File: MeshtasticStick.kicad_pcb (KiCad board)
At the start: 2 copper layers, 31 x 60 mm, 3 parts

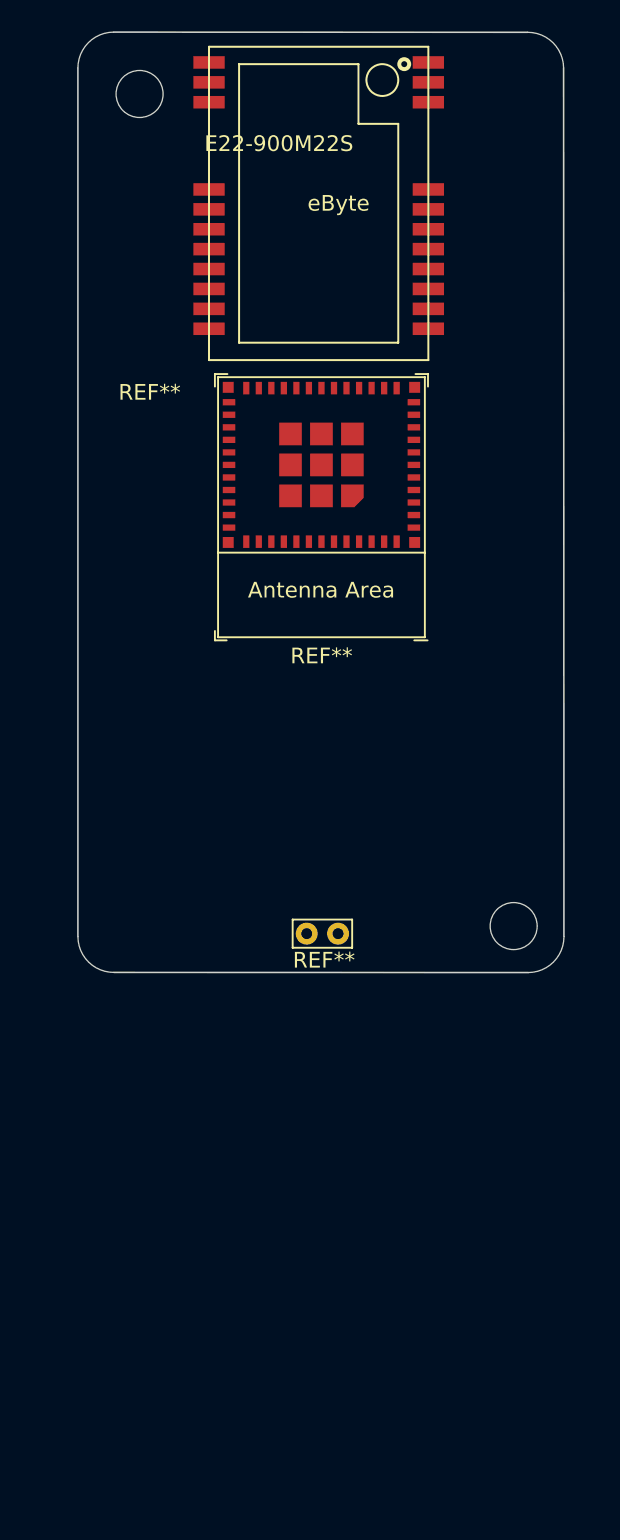
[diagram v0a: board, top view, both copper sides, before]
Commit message: ver1
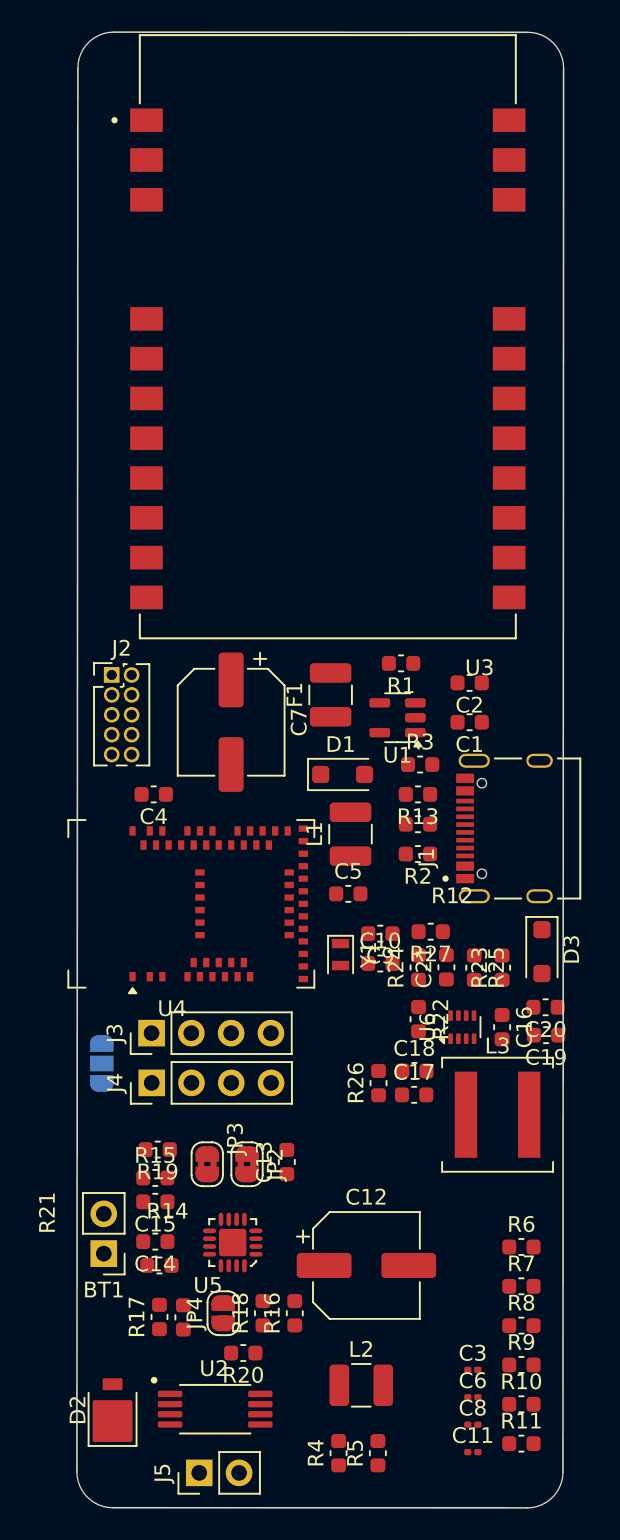
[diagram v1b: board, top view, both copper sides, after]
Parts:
- removed REF**: ESP32-PICO-MINI-02, PCM_Espressif:ESP32-PICO-MINI-02
- removed REF**: E22-900M22S, RF_Module:E22-900M22S
- removed REF**: TestPoint_Bridge_Pitch2.0mm_Drill0.7mm, TestPoint:TestPoint_Bridge_Pitch2.0mm_Drill0.7mm
- added BT1: Battery_Cell, Connector_PinHeader_2.54mm:PinHeader_1x02_P2.54mm_Vertical, F.Cu at (126.5, 146.8)
- added C1: 1uF, Capacitor_SMD:C_0603_1608Metric, F.Cu at (149.8, 112.9)
- added C10: 14p, Capacitor_SMD:C_0603_1608Metric, F.Cu at (144.1, 128.3)
- added C11: 1nF, Capacitor_SMD:C_0201_0603Metric, F.Cu at (150.0, 159.5)
- added C12: 47uF, Capacitor_SMD:CP_Elec_6.3x7.7, F.Cu at (143.3, 147.5)
- added C13: 10nF, Capacitor_SMD:C_0603_1608Metric, F.Cu at (138.2, 140.9)
- added C14: 4.7uF, Capacitor_SMD:C_0603_1608Metric, F.Cu at (129.8, 146.0)
- added C15: 1nF, Capacitor_SMD:C_0603_1608Metric, F.Cu at (129.8, 143.5)
- added C16: 0.1uF, Capacitor_SMD:C_0603_1608Metric, F.Cu at (151.9, 132.3)
- added C17: 10uF, Capacitor_SMD:C_0603_1608Metric, F.Cu at (146.3, 136.7)
- added C18: 0.1uF, Capacitor_SMD:C_0603_1608Metric, F.Cu at (146.3, 135.1)
- added C19: 22uF, Capacitor_SMD:C_0603_1608Metric, F.Cu at (154.7, 132.8)
- added C2: 1uF, Capacitor_SMD:C_0603_1608Metric, F.Cu at (149.8, 110.4)
- added C20: 22uF, Capacitor_SMD:C_0603_1608Metric, F.Cu at (154.7, 131.1)
- added C21: 22nF, Capacitor_SMD:C_0603_1608Metric, F.Cu at (148.4, 128.5)
- added C3: 1uF, Capacitor_SMD:C_0201_0603Metric, F.Cu at (150.0, 154.2)
- added C4: 4.7uF, Capacitor_SMD:C_0603_1608Metric, F.Cu at (129.7, 117.5)
- added C5: 4.7uF, Capacitor_SMD:C_0603_1608Metric, F.Cu at (142.1, 123.8)
- added C6: 1nF, Capacitor_SMD:C_0201_0603Metric, F.Cu at (150.0, 156.0)
- added C7: 100uF, Capacitor_SMD:CP_Elec_6.3x7.7, F.Cu at (134.6, 112.9)
- added C8: 10uF, Capacitor_SMD:C_0201_0603Metric, F.Cu at (150.0, 157.7)
- added C9: 14p, Capacitor_SMD:C_0603_1608Metric, F.Cu at (144.1, 126.4)
- added D1: MBR120VLSFT1G, Diode_SMD:D_SOD-123F, F.Cu at (141.7, 116.2)
- added D2: SMM4F5.0A, Diode_SMD:D_SMP_DO-220AA, F.Cu at (127.1, 156.8)
- added D3: MBR120VLSFT1G, Diode_SMD:D_SOD-123F, F.Cu at (154.5, 127.5)
- added F1: Fuse, Fuse:Fuse_1210_3225Metric, F.Cu at (141.0, 111.1)
- added J1: TYPE-C-31-M-12, TYPE-C-31-M-12 footprint:HRO_TYPE-C-31-M-12, F.Cu at (154.3, 119.7)
- added J2: Conn_02x05_Odd_Even, Connector_PinHeader_1.27mm:PinHeader_2x05_P1.27mm_Vertical, F.Cu at (127.0, 109.9)
- added J3: Conn_01x04, Connector_PinHeader_2.54mm:PinHeader_1x04_P2.54mm_Vertical, F.Cu at (129.5, 132.7)
- added J4: Conn_01x04, Connector_PinHeader_2.54mm:PinHeader_1x04_P2.54mm_Vertical, F.Cu at (129.6, 135.9)
- added J5: Conn_01x02, Connector_PinHeader_2.54mm:PinHeader_1x02_P2.54mm_Vertical, F.Cu at (132.6, 160.8)
- added JP1: SolderJumper_3_Bridged12, Jumper:SolderJumper-3_P1.3mm_Open_RoundedPad1.0x1.5mm, B.Cu at (126.4, 134.7)
- added JP2: Jumper_2_Bridged, Jumper:SolderJumper-2_P1.3mm_Bridged2Bar_RoundedPad1.0x1.5mm, F.Cu at (135.6, 141.1)
- added JP3: Jumper_2_Bridged, Jumper:SolderJumper-2_P1.3mm_Bridged2Bar_RoundedPad1.0x1.5mm, F.Cu at (133.1, 141.1)
- added JP4: Jumper_2_Open, Jumper:SolderJumper-2_P1.3mm_Open_RoundedPad1.0x1.5mm, F.Cu at (134.1, 150.6)
- added L1: 10uH, Inductor_SMD:L_1210_3225Metric, F.Cu at (142.2, 120.0)
- added L2: 10uH, Fuse:Fuse_1210_3225Metric, F.Cu at (142.9, 155.2)
- added L3: MDA4020-1R0M 6.8uH/8.5A/16mR, Inductor_SMD:L_Coilcraft_XAL6060-XXX, F.Cu at (151.6, 137.9)
- added R1: 10K, Capacitor_SMD:C_0603_1608Metric, F.Cu at (145.5, 109.1)
- added R10: 2.2M, Capacitor_SMD:C_0603_1608Metric, F.Cu at (153.1, 156.4)
- added R11: 820K, Capacitor_SMD:C_0603_1608Metric, F.Cu at (153.1, 158.9)
- added R12: 27R, Capacitor_SMD:C_0603_1608Metric, F.Cu at (146.5, 119.4)
- added R13: 27R, Capacitor_SMD:C_0603_1608Metric, F.Cu at (146.5, 117.5)
- added R14: 3.3K, Capacitor_SMD:C_0603_1608Metric, F.Cu at (130.0, 147.5)
- added R15: 1K, Capacitor_SMD:C_0603_1608Metric, F.Cu at (129.8, 142.0)
- added R16: 24K, Capacitor_SMD:C_0603_1608Metric, F.Cu at (138.7, 150.6)
- added R17: DNM, Capacitor_SMD:C_0603_1608Metric, F.Cu at (130.0, 150.8)
- added R18: DNM, Capacitor_SMD:C_0603_1608Metric, F.Cu at (136.7, 150.6)
- added R19: 470R, Capacitor_SMD:C_0603_1608Metric, F.Cu at (129.9, 140.1)
- added R2: 5.1K, Capacitor_SMD:C_0603_1608Metric, F.Cu at (146.5, 121.3)
- added R20: DNM, Capacitor_SMD:C_0603_1608Metric, F.Cu at (135.4, 153.1)
- added R21: DNM, Capacitor_SMD:C_0603_1608Metric, F.Cu at (131.6, 150.9)
- added R22: 90.9K, Capacitor_SMD:C_0603_1608Metric, F.Cu at (146.6, 131.8)
- added R23: 68K, Capacitor_SMD:C_0603_1608Metric, F.Cu at (151.9, 128.5)
- added R24: 10K, Capacitor_SMD:C_0603_1608Metric, F.Cu at (146.6, 128.5)
- added R25: 18K, Capacitor_SMD:C_0603_1608Metric, F.Cu at (150.1, 128.5)
- added R26: 100K, Capacitor_SMD:C_0603_1608Metric, F.Cu at (144.0, 135.9)
- added R27: 10K, Capacitor_SMD:C_0603_1608Metric, F.Cu at (147.4, 126.2)
- added R3: 5.1K, Capacitor_SMD:C_0603_1608Metric, F.Cu at (146.7, 115.6)
- added R4: 1K, Capacitor_SMD:C_0603_1608Metric, F.Cu at (141.5, 159.5)
- added R5: 1K, Capacitor_SMD:C_0603_1608Metric, F.Cu at (144.0, 159.5)
- added R6: 1K, Capacitor_SMD:C_0603_1608Metric, F.Cu at (153.1, 146.4)
- added R7: DNM, Capacitor_SMD:C_0603_1608Metric, F.Cu at (153.1, 148.9)
- added R8: 0R, Capacitor_SMD:C_0603_1608Metric, F.Cu at (153.1, 151.4)
- added R9: 0R, Capacitor_SMD:C_0603_1608Metric, F.Cu at (153.1, 153.9)
- added U1: AP2112K-3.3, Package_TO_SOT_SMD:SOT-23-5, F.Cu at (145.2, 112.6)
- added U2: SPV1040T, STMicroelectronics SPV1040T:SOP65P640X120-8N, F.Cu at (133.6, 156.7)
- added U3: E22-900M30S, E22-900M30S footprint:XCVR_E22-900M30S, F.Cu at (140.8, 88.3)
- added U4: MDBT50Q-P1MV2, RF_Module:Raytac_MDBT50Q, F.Cu at (132.1, 124.5)
- added U5: L6924D, L6924D footprint:QFN50P300X300X100-17N, F.Cu at (134.7, 146.1)
- added U6: MP2338GTL, Package_TO_SOT_SMD:SOT-583-8, F.Cu at (149.4, 132.3)
- added Y1: Crystal, Crystal:Crystal_SMD_2012-2Pin_2.0x1.2mm, F.Cu at (141.6, 127.7)
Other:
- board size 31 x 60 mm -> 31.1 x 94.2 mm
